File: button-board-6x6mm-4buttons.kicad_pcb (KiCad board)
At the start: 2 copper layers, 52 x 20 mm, 23 parts, among them J1 Conn_02x03_Counter_Clockwise, SW1 SW_Push, SW2 SW_Push, SW3 SW_Push, SW4 SW_Push

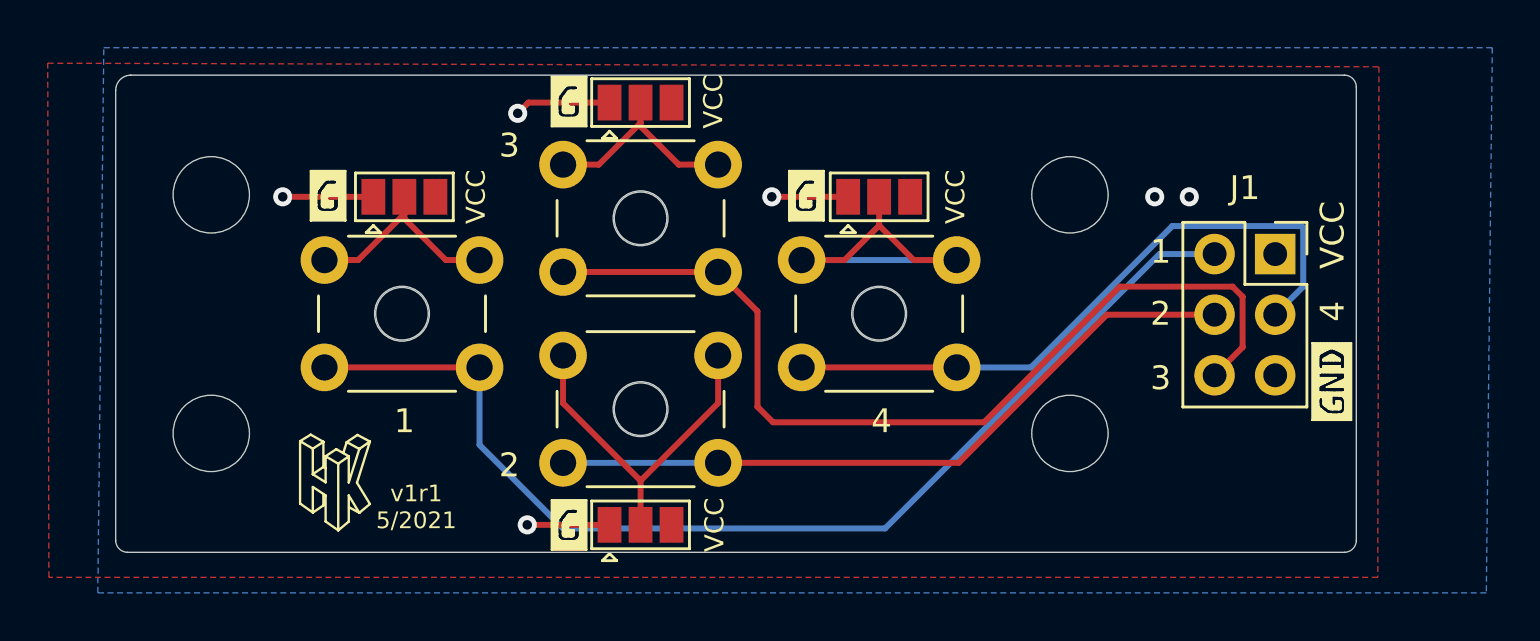
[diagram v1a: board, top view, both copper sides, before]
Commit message: update to v1r1
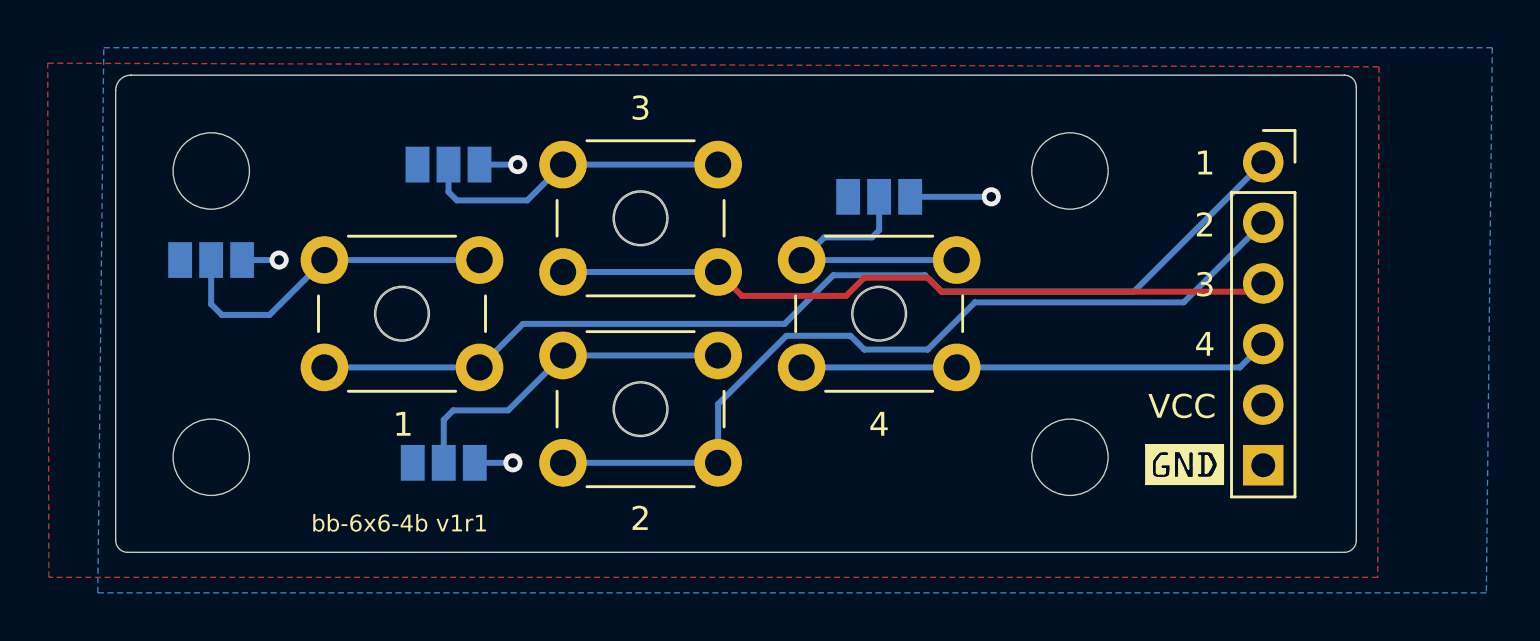
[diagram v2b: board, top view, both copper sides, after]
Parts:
- removed the REF** at (55.5, 33.1)
- removed the REF** at (55.5, 50.9)
- added REF**: SYM_G_SilkScreen_Front, zytzeiche:SYM_G_SilkScreen_Front, B.Cu at (47.4, 35.8)
- added REF**: SYM_G_SilkScreen_Front, zytzeiche:SYM_G_SilkScreen_Front, B.Cu at (47.1, 48.3)
- J1: value Conn_02x03_Counter_Clockwise -> Conn_01x06_Male; footprint Connector_PinSocket_2.54mm:PinSocket_2x03_P2.54mm_Vertical -> Connector_PinSocket_2.54mm:PinSocket_1x06_P2.54mm_Vertical
- JP1, JP2, JP3, JP4, REF** (x2): moved to B.Cu
- moved JP2 8.65 mm to (50.2, 48.2)
- moved JP1 8.52 mm to (40.5, 39.8)
- moved JP3 8.46 mm to (50.5, 35.8)
- moved REF** 8.40 mm to (37.5, 39.8), turned to 180 degrees
- moved REF** 7.14 mm to (81.2, 48.4), turned to 0 degrees
- moved REF** 6.87 mm to (81.5, 48.4), turned to 0 degrees
- moved J1 3.88 mm to (84.6, 35.6)
- moved H1 1.00 mm to (40.5, 36.0)
- moved H5 1.00 mm to (76.5, 36.0)
- moved H7 1.00 mm to (40.5, 48.0)
- moved H8 1.00 mm to (76.5, 48.0)
- turned REF** to 180 degrees
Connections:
- J1 pad 1: VCC -> Net-(J1-Pad1)
- J1 pad 5: GND -> VCC
- J1 pad 6: Net-(J1-Pad6) -> GND
- SW1 pad 2: Net-(J1-Pad2) -> Net-(J1-Pad1)
- SW2 pad 2: Net-(J1-Pad4) -> Net-(J1-Pad2)
- SW3 pad 2: Net-(J1-Pad6) -> Net-(J1-Pad3)
- SW4 pad 2: Net-(J1-Pad3) -> Net-(J1-Pad4)
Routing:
- net Net-(J1-Pad1): track 0.00 -> 43.5 mm
- net Net-(J1-Pad6): track 39.7 -> 0.00 mm
- net GND: track 15.0 -> 0.00 mm, vias 6 -> 0
- net Net-(J1-Pad2): track 46.8 -> 35.4 mm
- net Net-(J1-Pad4): track 29.9 -> 19.8 mm
- net VCC: track 0.00 -> 8.25 mm, vias 0 -> 4
- net Net-(JP1-Pad2): track 9.65 -> 14.2 mm
- net Net-(JP3-Pad2): track 8.89 -> 13.2 mm
- net Net-(JP4-Pad2): track 15.4 -> 11.7 mm
- net Net-(J1-Pad3): track 27.6 -> 30.5 mm
- net Net-(JP2-Pad2): track 15.0 -> 14.4 mm
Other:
- board text added: "- 3 buttons (6x6) - 52x20mm - holes d=3.2mm, distance=36mm and 12mm"
- board text added: "4 buttons (6x6), 52x20mm, M3 holes d=3.2mm, distance=36/12mm"
- board text added: "Btn1"
- board text added: "Btn2"
- board text added: "Btn3"
- board text added: "Btn4"
- board text added: "M3"
- board text added: "bb-6x6-4b v1r1"
- board text removed: "- 3 buttons (6x6) - 52x20mm - holes d=3.2mm, distance=36mm and 10mm"
- board text removed: "3 buttons (6x6), 52x12mm, holes d=3.3mm, distance=36/10mm"
